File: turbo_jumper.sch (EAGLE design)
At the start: 9 parts, among them K1 351, X1 E74, X2 P-remote

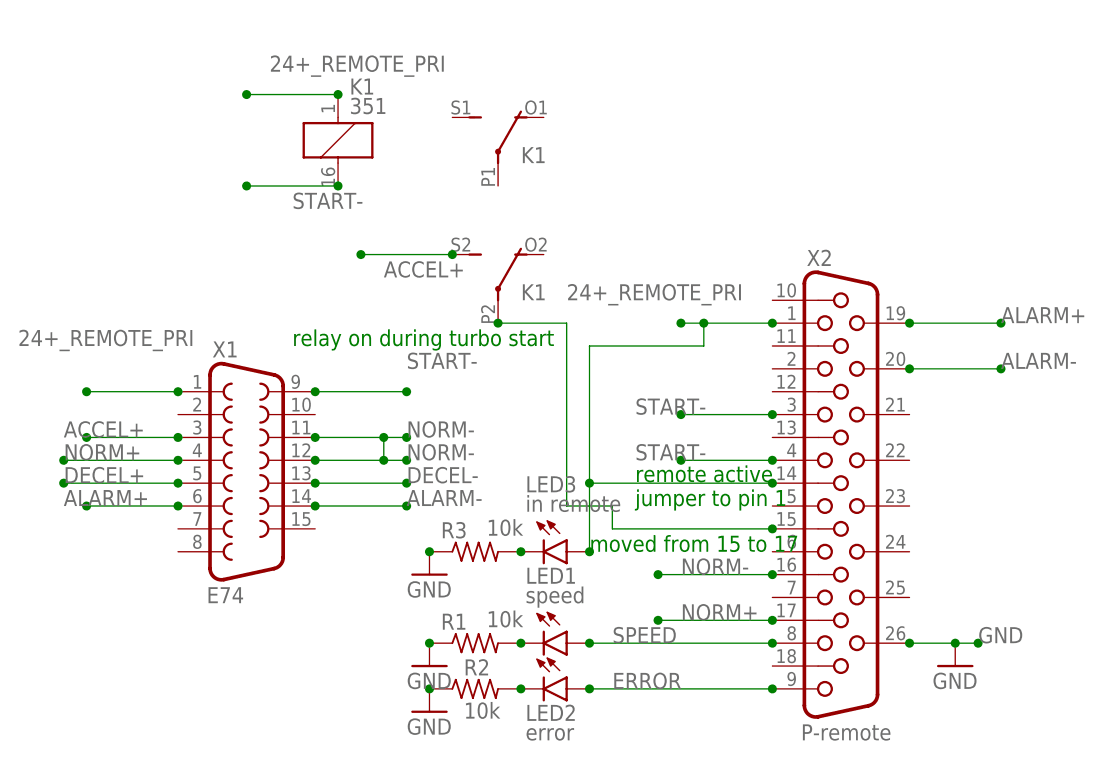
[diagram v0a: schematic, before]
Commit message: up
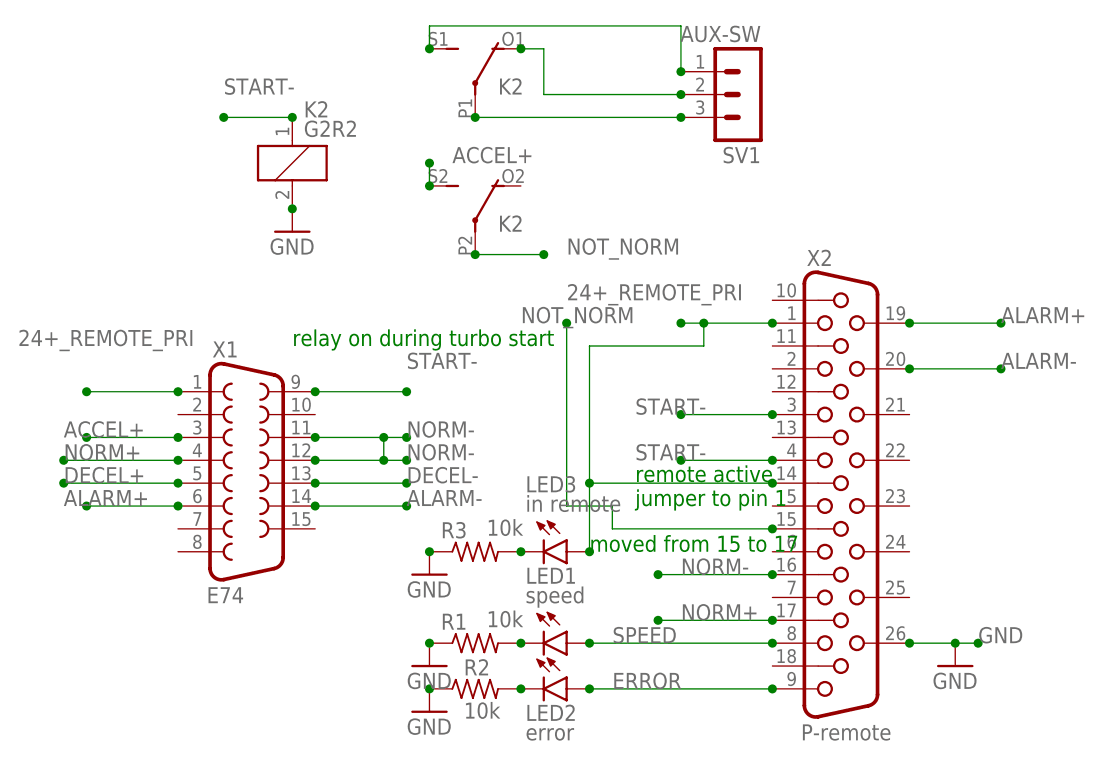
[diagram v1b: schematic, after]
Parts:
- removed K1: 351, relay:351
- added K2: G2R2, relay:G2R2
- added SV1: AUX-SW, con-lstb:MA03-1
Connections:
- new net N$5: K22.O, SV1.2
- new net N$6: K22.S, SV1.1
- new net NOT_NORM: K23.P, X2.15
- net 24+_REMOTE_PRI: no longer K11.1
- net ACCEL+: now also K23.S; no longer K13.S
- net GND: now also K21.2
- net N$1: now also K22.P, SV1.3; no longer K13.P, X2.15
- net START-: now also K21.1; no longer K11.2
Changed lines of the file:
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@@
 <part name="R3" library="rcl" library_urn="urn:adsk.eagle:library:334" deviceset="R-US_" device="M1206" package3d_urn="urn:adsk.eagle:package:23566/2" value="10k"/>
 <part name="GND4" library="supply1" library_urn="urn:adsk.eagle:library:371" deviceset="GND" device=""/>
-<part name="K1" library="relay" library_urn="urn:adsk.eagle:library:339" deviceset="351" device="" package3d_urn="urn:adsk.eagle:package:24300/1"/>
+<part name="K2" library="relay" library_urn="urn:adsk.eagle:library:339" deviceset="G2R2" device="" package3d_urn="urn:adsk.eagle:package:24328/1"/>
+<part name="GND6" library="supply1" library_urn="urn:adsk.eagle:library:371" deviceset="GND" device=""/>
+<part name="SV1" library="con-lstb" library_urn="urn:adsk.eagle:library:162" deviceset="MA03-1" device="" package3d_urn="urn:adsk.eagle:package:8339/1" value="AUX-SW"/>
 </parts>
 <sheets>
@@
 <attribute name="VALUE" x="40.64" y="45.72" size="1.778" layer="96"/>
 </instance>
-<instance part="K1" gate="1" x="33.02" y="96.52" smashed="yes">
-<attribute name="VALUE" x="34.29" y="99.441" size="1.778" layer="96"/>
-<attribute name="PART" x="34.29" y="101.6" size="1.778" layer="95"/>
-</instance>
-<instance part="K1" gate="2" x="50.8" y="93.98" smashed="yes">
-<attribute name="PART" x="53.34" y="93.98" size="1.778" layer="95"/>
-</instance>
-<instance part="K1" gate="3" x="50.8" y="78.74" smashed="yes">
-<attribute name="PART" x="53.34" y="78.74" size="1.778" layer="95"/>
+<instance part="K2" gate="1" x="27.94" y="93.98" smashed="yes">
+<attribute name="VALUE" x="29.21" y="96.901" size="1.778" layer="96"/>
+<attribute name="PART" x="29.21" y="99.06" size="1.778" layer="95"/>
+</instance>
+<instance part="K2" gate="2" x="48.26" y="101.6" smashed="yes">
+<attribute name="PART" x="50.8" y="101.6" size="1.778" layer="95"/>
+</instance>
+<instance part="K2" gate="3" x="48.26" y="86.36" smashed="yes">
+<attribute name="PART" x="50.8" y="86.36" size="1.778" layer="95"/>
+</instance>
+<instance part="GND6" gate="1" x="27.94" y="86.36" smashed="yes">
+<attribute name="VALUE" x="25.4" y="83.82" size="1.778" layer="96"/>
+</instance>
+<instance part="SV1" gate="G$1" x="78.74" y="101.6" smashed="yes" rot="R180">
+<attribute name="VALUE" x="80.01" y="109.22" size="1.778" layer="96" rot="R180"/>
+<attribute name="NAME" x="80.01" y="95.758" size="1.778" layer="95" rot="R180"/>
 </instance>
 </instances>
@@
 <junction x="60.96" y="58.42"/>
 </segment>
-<segment>
-<wire x1="33.02" y1="101.6" x2="22.86" y2="101.6" width="0.1524" layer="91"/>
-<pinref part="K1" gate="1" pin="1"/>
-<label x="25.4" y="104.14" size="1.778" layer="95"/>
-<junction x="33.02" y="101.6"/>
-<junction x="22.86" y="101.6"/>
-</segment>
 </net>
 <net name="START-" class="0">
@@
 </segment>
 <segment>
-<wire x1="22.86" y1="91.44" x2="33.02" y2="91.44" width="0.1524" layer="91"/>
-<pinref part="K1" gate="1" pin="2"/>
-<label x="27.94" y="88.9" size="1.778" layer="95"/>
-<junction x="33.02" y="91.44"/>
-<junction x="22.86" y="91.44"/>
+<wire x1="20.32" y1="99.06" x2="27.94" y2="99.06" width="0.1524" layer="91"/>
+<pinref part="K2" gate="1" pin="1"/>
+<label x="20.32" y="101.6" size="1.778" layer="95"/>
+<junction x="20.32" y="99.06"/>
+<junction x="27.94" y="99.06"/>
 </segment>
 </net>
@@
 </segment>
 <segment>
-<wire x1="45.72" y1="83.82" x2="35.56" y2="83.82" width="0.1524" layer="91"/>
-<pinref part="K1" gate="3" pin="S"/>
-<label x="38.1" y="81.28" size="1.778" layer="95"/>
-<junction x="45.72" y="83.82"/>
-<junction x="35.56" y="83.82"/>
+<wire x1="43.18" y1="91.44" x2="43.18" y2="93.98" width="0.1524" layer="91"/>
+<pinref part="K2" gate="3" pin="S"/>
+<label x="45.72" y="93.98" size="1.778" layer="95"/>
+<junction x="43.18" y="91.44"/>
+<junction x="43.18" y="93.98"/>
 </segment>
 </net>
@@
 <junction x="43.18" y="50.8"/>
 </segment>
+<segment>
+<pinref part="K2" gate="1" pin="2"/>
+<pinref part="GND6" gate="1" pin="GND"/>
+<junction x="27.94" y="88.9"/>
+</segment>
 </net>
 <net name="ERROR" class="0">
@@
 </segment>
 </net>
-<net name="N$1" class="0">
-<segment>
-<pinref part="K1" gate="3" pin="P"/>
-<wire x1="50.8" y1="76.2" x2="58.42" y2="76.2" width="0.1524" layer="91"/>
+<net name="NOT_NORM" class="0">
+<segment>
 <wire x1="58.42" y1="76.2" x2="58.42" y2="55.88" width="0.1524" layer="91"/>
 <pinref part="X2" gate="G$1" pin="15"/>
@@
 <wire x1="63.5" y1="53.34" x2="63.5" y2="55.88" width="0.1524" layer="91"/>
 <wire x1="63.5" y1="55.88" x2="58.42" y2="55.88" width="0.1524" layer="91"/>
-<junction x="50.8" y="76.2"/>
 <junction x="81.28" y="53.34"/>
-</segment>
-</net>
+<label x="53.34" y="76.2" size="1.778" layer="95"/>
+<junction x="58.42" y="76.2"/>
+</segment>
+<segment>
+<wire x1="48.26" y1="83.82" x2="55.88" y2="83.82" width="0.1524" layer="91"/>
+<pinref part="K2" gate="3" pin="P"/>
+<label x="58.42" y="83.82" size="1.778" layer="95"/>
+<junction x="48.26" y="83.82"/>
+<junction x="55.88" y="83.82"/>
+</segment>
+</net>
+<net name="N$1" class="0">
+<segment>
+<pinref part="K2" gate="2" pin="P"/>
+<pinref part="SV1" gate="G$1" pin="3"/>
+<wire x1="48.26" y1="99.06" x2="71.12" y2="99.06" width="0.1524" layer="91"/>
+<junction x="48.26" y="99.06"/>
+<junction x="71.12" y="99.06"/>
+</segment>
+</net>
+<net name="N$5" class="0">
+<segment>
+<pinref part="K2" gate="2" pin="O"/>
+<wire x1="53.34" y1="106.68" x2="55.88" y2="106.68" width="0.1524" layer="91"/>
+<wire x1="55.88" y1="106.68" x2="55.88" y2="101.6" width="0.1524" layer="91"/>
+<pinref part="SV1" gate="G$1" pin="2"/>
+<wire x1="55.88" y1="101.6" x2="71.12" y2="101.6" width="0.1524" layer="91"/>
+<junction x="53.34" y="106.68"/>
+<junction x="71.12" y="101.6"/>
+</segment>
+</net>
+<net name="N$6" class="0">
+<segment>
+<pinref part="SV1" gate="G$1" pin="1"/>
+<wire x1="71.12" y1="104.14" x2="71.12" y2="109.22" width="0.1524" layer="91"/>
+<wire x1="71.12" y1="109.22" x2="43.18" y2="109.22" width="0.1524" layer="91"/>
+<pinref part="K2" gate="2" pin="S"/>
+<wire x1="43.18" y1="109.22" x2="43.18" y2="106.68" width="0.1524" layer="91"/>
+<junction x="43.18" y="106.68"/>
+<junction x="71.12" y="104.14"/>
+</segment>
+</net>
